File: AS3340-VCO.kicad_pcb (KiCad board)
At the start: 2 copper layers, 71 x 133.2 mm, 72 parts, among them J1 1V/OCT_IN, J10 SAWTOOTH_OUT, J11 TRIANGLE_OUT, J12 EURO_PWR_2x5, J2 1V/OCT_OUT, J3 CV2_INPUT, J4 EXT_PWM_CTRL_IN, J5 POS_HARD_SYNC_IN, J6 NEG_HARD_SYNC_IN, J7 SOFT_SYNC_IN, J8 FM_IN, J9 SQUARE_OUT, SW1 SW_SPDT, U1 TL074, U2 AS3340

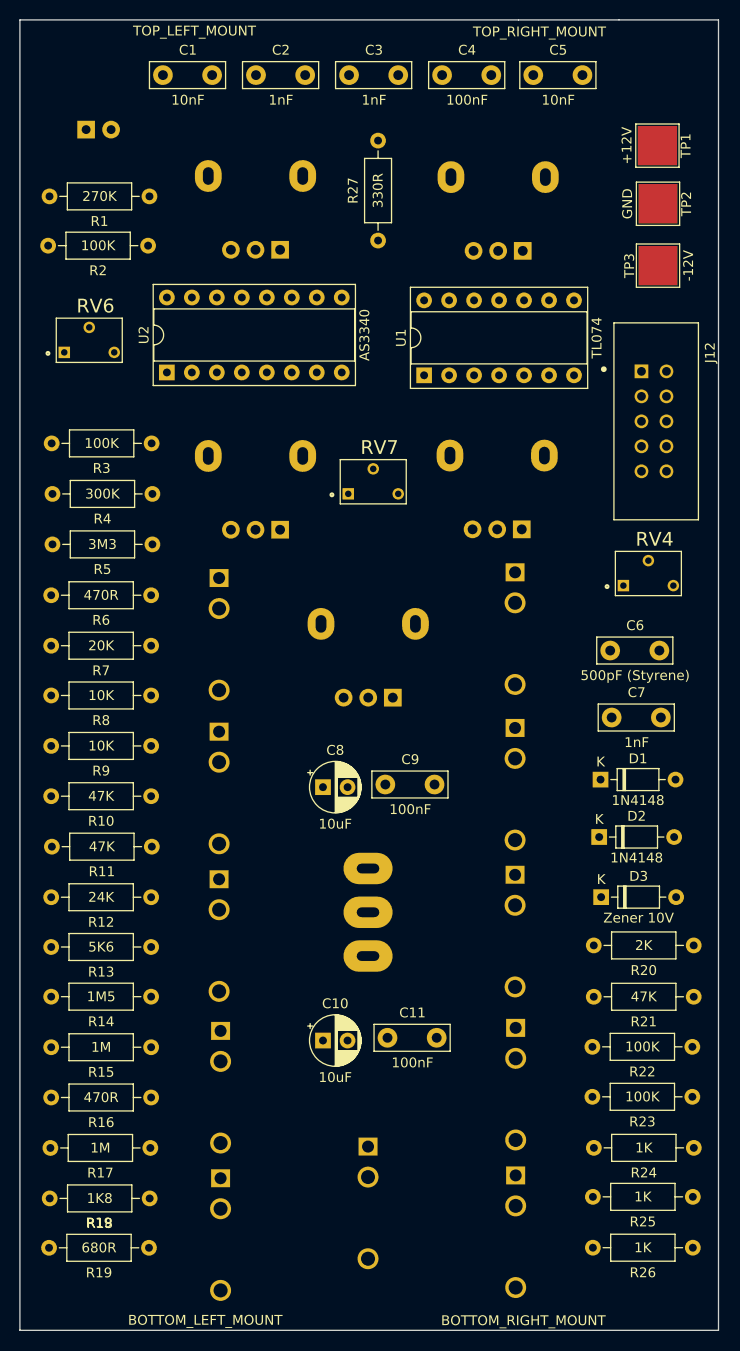
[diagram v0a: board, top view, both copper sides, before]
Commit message: Revv. 2
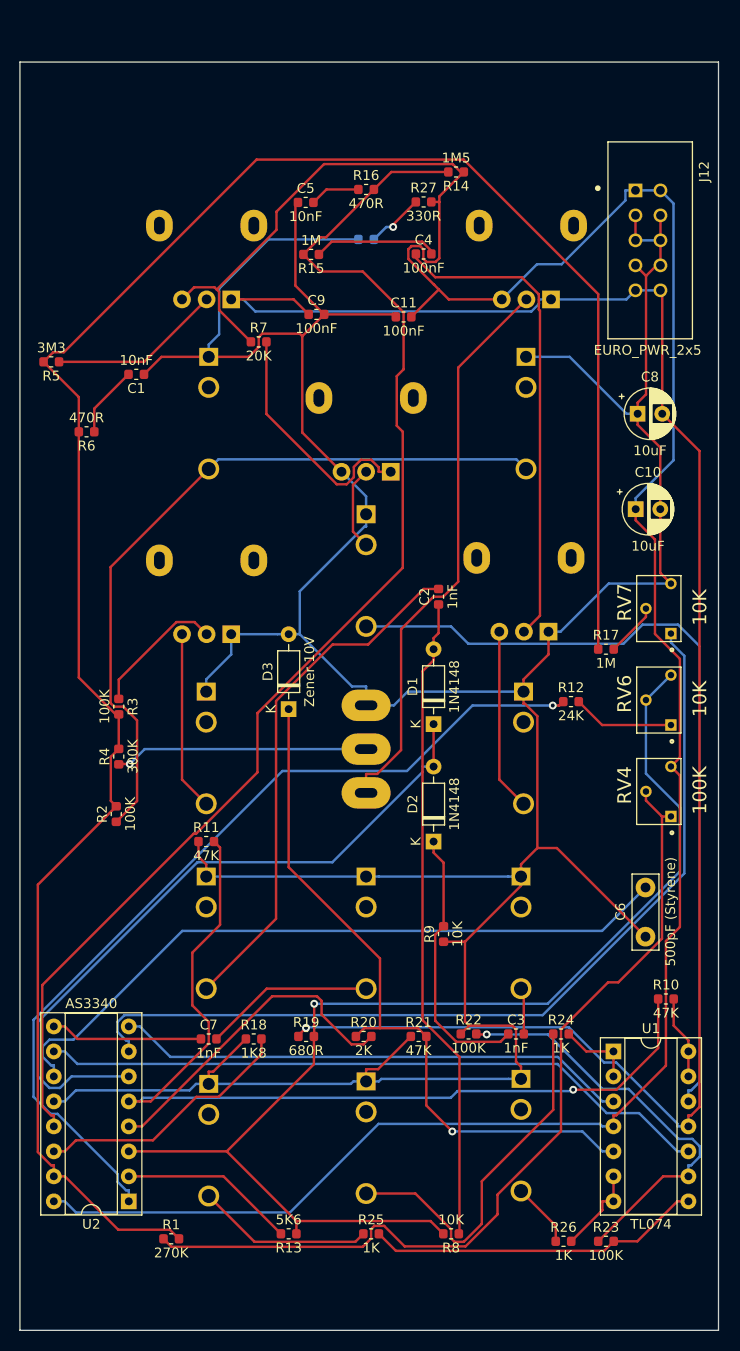
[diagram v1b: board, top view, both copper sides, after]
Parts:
- removed TP1: +12V, Seattle_Synths:TestPoint_Pad_4.0x4.0mm
- removed TP2: GND, Seattle_Synths:TestPoint_Pad_4.0x4.0mm
- removed TP3: -12V, Seattle_Synths:TestPoint_Pad_4.0x4.0mm
- C1, C11, C2, C3, C4, C5, C7, C9: footprint Seattle_Synths:C_Disc_D7.5mm_W2.5mm_P5.00mm -> Seattle_Synths:C_0603_1608Metric
- D4: footprint Seattle_Synths:LED_D5.0mm -> Seattle_Synths:D_0603_1608Metric
- R1, R10, R11, R12, R13, R14, R15, R16, R17, R18, R19, R2, R20, R21, R22, R23, R24, R25, R26, R27, R3, R4, R5, R6, R7, R8, R9: footprint Seattle_Synths:R_Axial_DIN0207_L6.3mm_D2.5mm_P10.16mm_Horizontal -> Seattle_Synths:R_0603_1608Metric
- RV1: value 100K -> 100K (Fine)
- RV2: value 100K -> 100K (CV2)
- RV3: value 100K -> 100K (PWM)
- RV5: value 100K -> 100K (Pitch)
- RV8: value 100K -> 100K (FM)
- moved R1 106.7 mm to (126.0, 143.3)
- moved C3 98.9 mm to (161.0, 122.4)
- moved R16 97.7 mm to (145.8, 36.6)
- moved R14 93.4 mm to (154.9, 34.8), turned to 180 degrees
- moved R15 84.8 mm to (140.2, 43.2), turned to 180 degrees
- moved U2 84.4 mm to (121.7, 139.4), turned to 180 degrees
- moved R17 75.9 mm to (170.2, 83.3)
- moved C11 73.3 mm to (149.6, 49.5)
- moved U1 71.4 mm to (170.9, 124.2), turned to 0 degrees
- moved RV6 68.9 mm to (176.8, 88.5), turned to 90 degrees
- moved R8 68.2 mm to (154.4, 142.7), turned to 180 degrees
- moved R10 65.8 mm to (176.3, 118.9)
- moved C10 62.7 mm to (173.2, 69.1)
- moved R2 58.2 mm to (120.4, 100.1), turned to 90 degrees
- moved R12 56.5 mm to (166.6, 88.6)
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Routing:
- net GND: track 0.00 -> 388.5 mm
- net +12V: track 0.00 -> 259.4 mm
- net /FREQ_CTRL: track 0.00 -> 212.9 mm
- net -12V: track 0.00 -> 185.5 mm, vias 0 -> 1
- net /LINEAR_FM: track 0.00 -> 130.1 mm
- net Net-(R13-Pad1): track 0.00 -> 120.6 mm, vias 0 -> 1
- net /PWM: track 0.00 -> 94.3 mm, vias 0 -> 1
- net Net-(RV7-Pad1): track 0.00 -> 92.5 mm
- net Net-(R12-Pad1): track 0.00 -> 90.3 mm, vias 0 -> 1
- net Net-(R1-Pad1): track 0.00 -> 90.1 mm
- net Net-(J4-PadT): track 0.00 -> 83.2 mm
- net Net-(J1-PadT): track 0.00 -> 75.6 mm
- net Net-(D3-Pad1): track 0.00 -> 72.1 mm, vias 0 -> 1
- net Net-(C6-Pad2): track 0.00 -> 71.7 mm
- net /HARD_SYNC: track 0.00 -> 71.4 mm
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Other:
- board size 71 x 133.2 mm -> 71 x 128.9 mm
